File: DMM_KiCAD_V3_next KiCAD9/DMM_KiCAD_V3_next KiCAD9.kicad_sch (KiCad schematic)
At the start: 70 parts, among them J1 Conn_01x07_Pin, J10 ANALOG, J11 I_Input, J12 Conn_01x02_Pin, J13 DIGITAL1, J14 Barrel_Jack, J15 Barrel_Jack, J16 Conn_01x01_Socket, J17 Conn_01x01_Socket, J2 MicoSD, J3 Conn_01x07_Pin, J5 POWER2, J6 POWER1, J7 Conn_01x02_Pin, J8 DIGITAL2, J9 Out to Screen, Q1 MMBT3904, Q2 SI2302 MOSFET, Q6 BSS138, Q7 BSS138, Q8 SI2302 MOSFET, SW1 SW_Push, SW2 SW_Push, SW3 SW_SPDT, SW4 SW_Push, U1 LM317_TO-220, U10 LM4040DBZ-2.5, U11 LM4040DBZ-5, U3 ADS1115IDGS, U7 MAX1683, U9 TPS613222ADBV

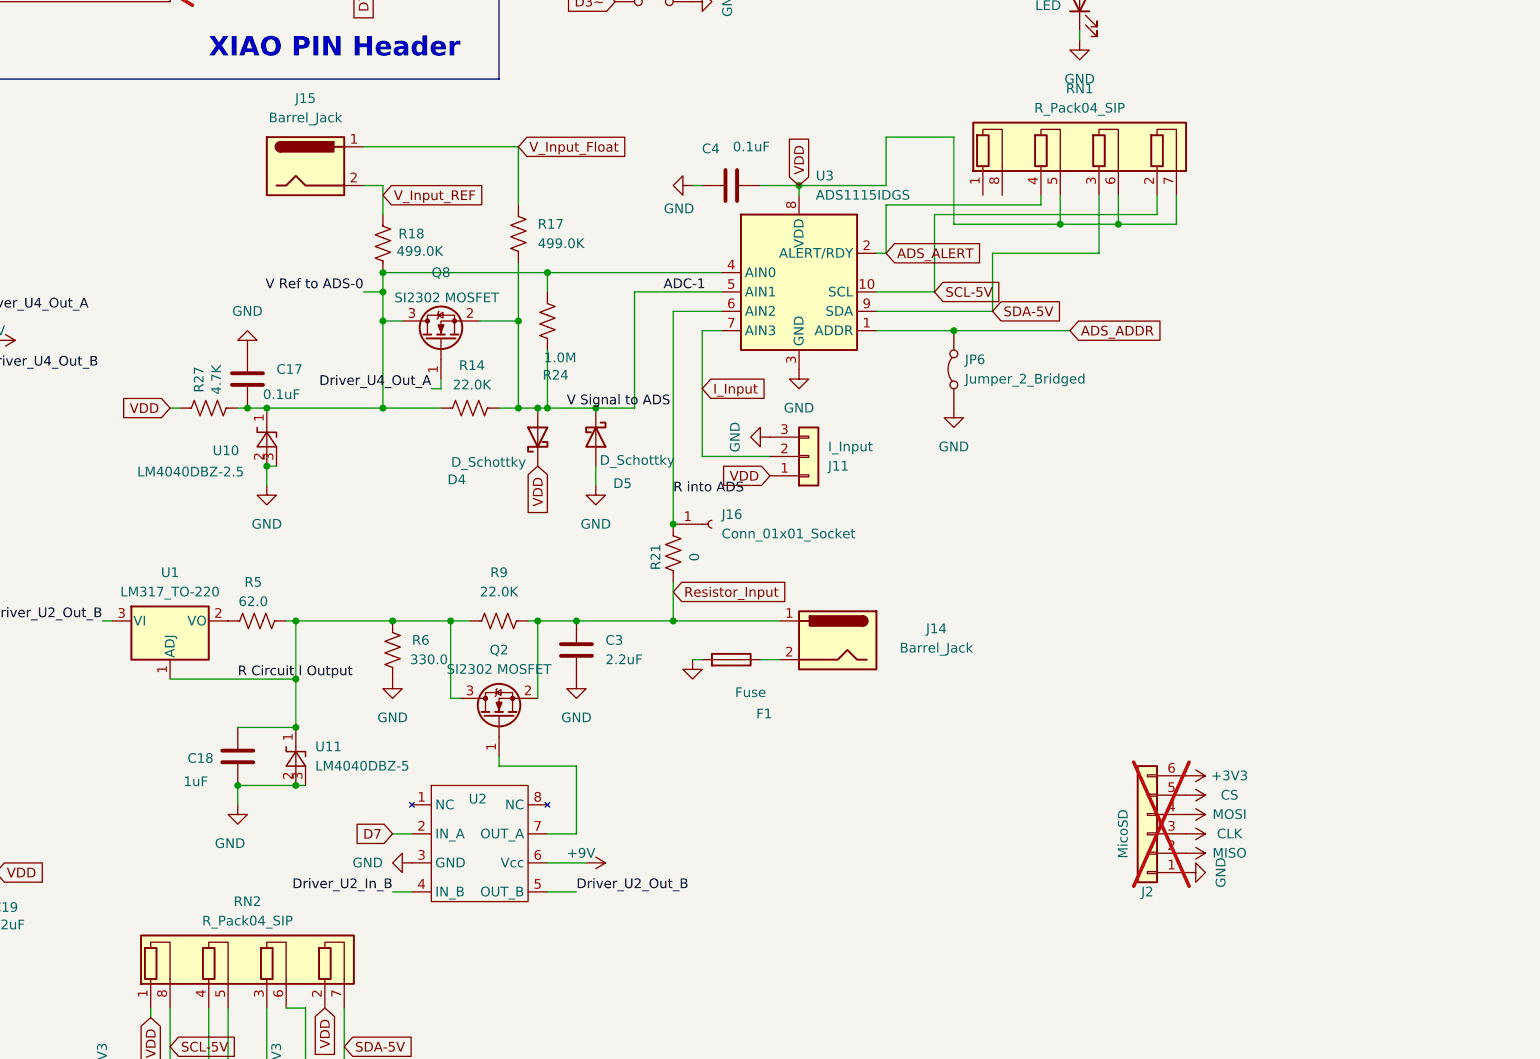
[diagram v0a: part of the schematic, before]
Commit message: Finishing the next PCB version
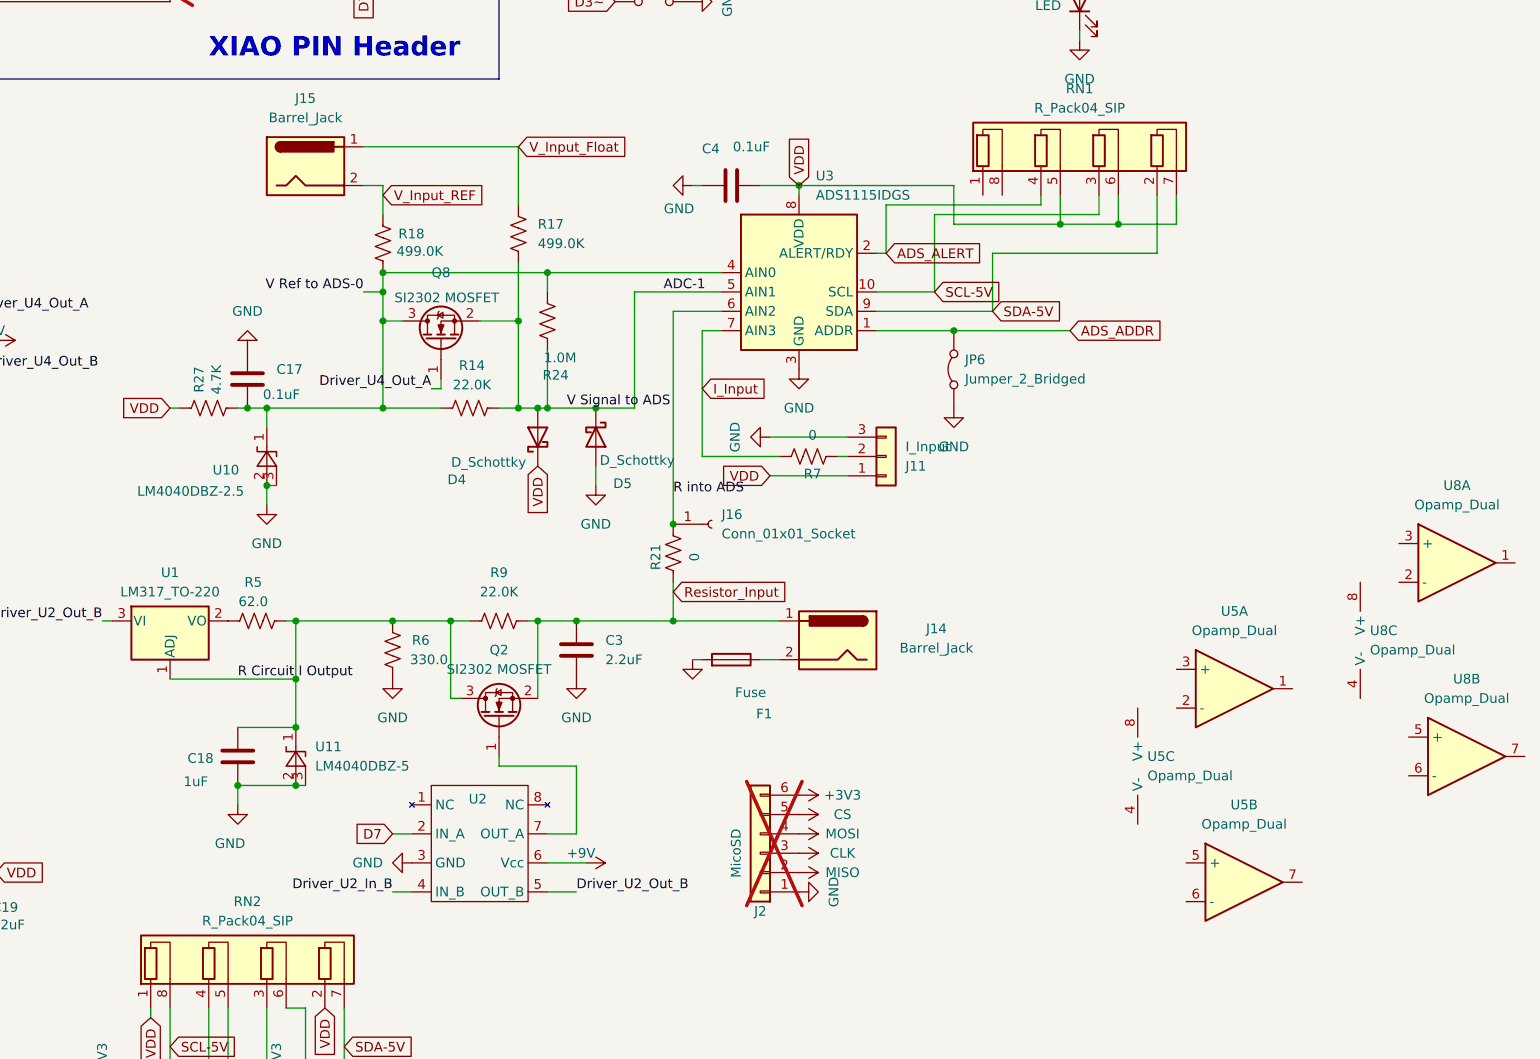
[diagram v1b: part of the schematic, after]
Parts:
- added R7: 0, Resistor_SMD:R_0805_2012Metric_Pad1.20x1.40mm_HandSolder, symbol Device:R_US
- added U5, U8: Opamp_Dual, Package_SO:SOIC-8_3.9x4.9mm_P1.27mm, symbol Device:Opamp_Dual
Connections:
- net I_Input: now also R7.1; no longer J11.2 (Pin_2)
- net SCL-5V: now also RN1.3 (R3.1); no longer RN1.2 (R4.1)
- net SDA-5V: now also RN1.2 (R4.1); no longer RN1.3 (R3.1)
- new net: J11.2 (Pin_2), R7.2
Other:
- moved on the sheet: J11, J2, U10
